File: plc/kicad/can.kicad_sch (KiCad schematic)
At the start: 1 part, among them CN2 DB2ERC-3.81-3P

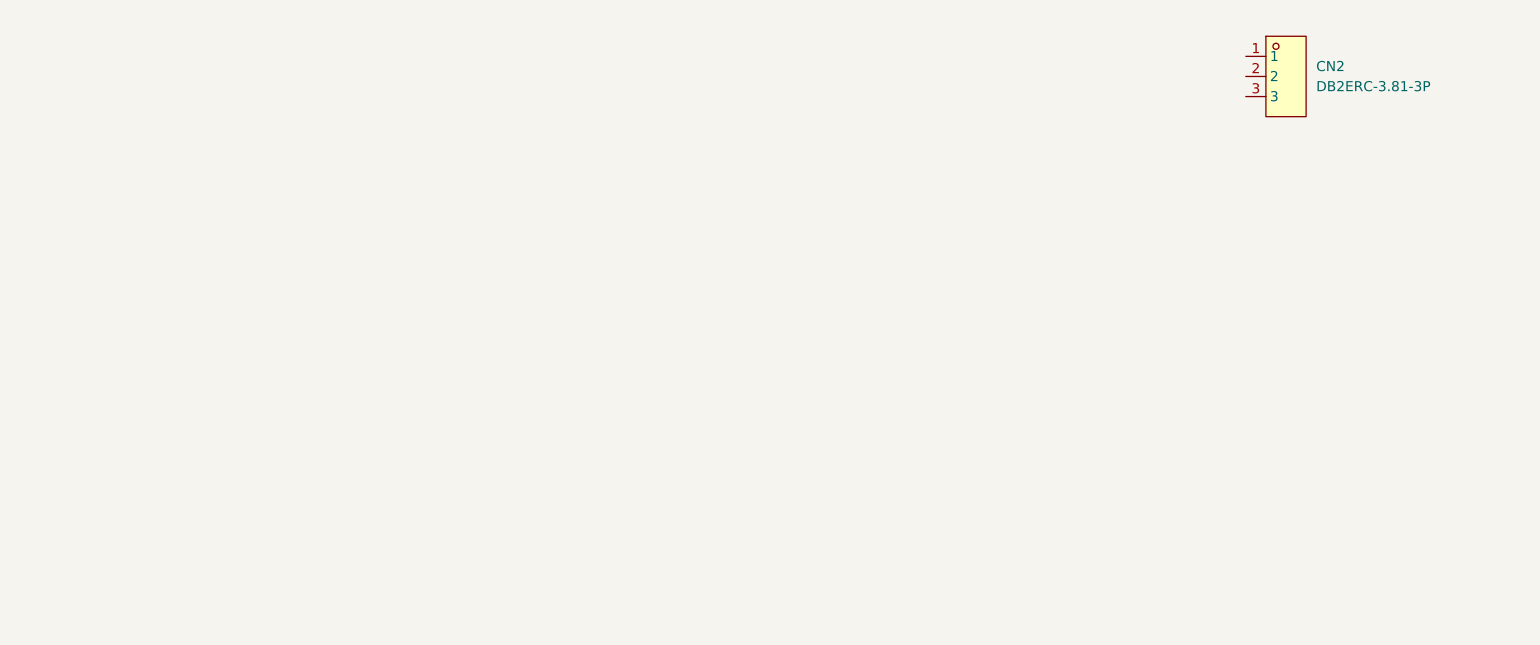
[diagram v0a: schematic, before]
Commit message: Added CAN circuit
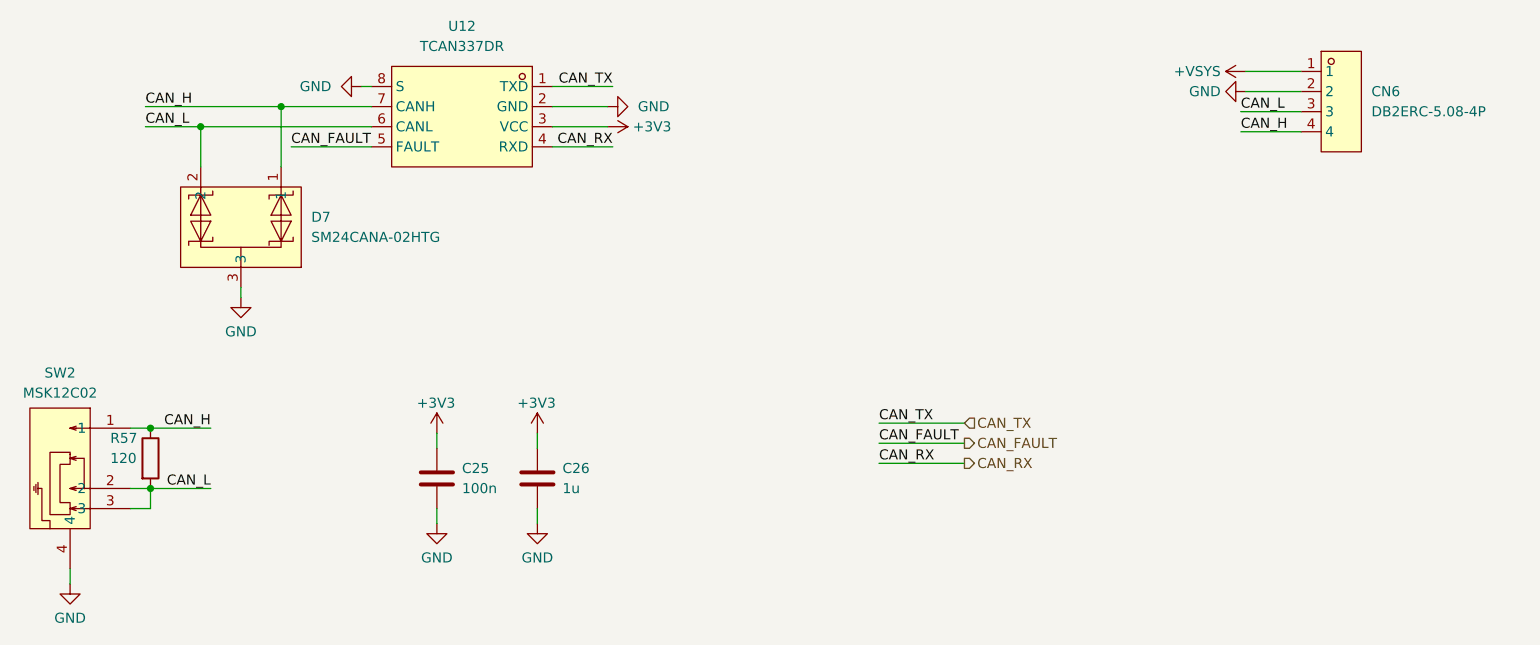
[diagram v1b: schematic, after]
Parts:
- removed CN2: DB2ERC-3.81-3P, LibrePLC32:CONN-TH_3P-P3.81_DB2ERC-3.81-3P, symbol LibrePLC32:DB2ERC-3.81-3P
- added C25: 100n, Capacitor_SMD:C_0805_2012Metric, symbol Device:C
- added C26: 1u, Capacitor_SMD:C_0805_2012Metric, symbol Device:C
- added CN6: DB2ERC-5.08-4P, LibrePLC32:CONN-TH_4P-P5.08_DB2ERC-5.08-4P, symbol LibrePLC32:DB2ERC-5.08-4P
- added D7: SM24CANA-02HTG, LibrePLC32:SOT-23_L2.9-W1.3-P1.90-LS2.4-BR, symbol LibrePLC32:SM24CANA-02HTG
- added R57: 120, Resistor_SMD:R_0805_2012Metric, symbol Device:R
- added SW2: MSK12C02, LibrePLC32:SW-TH_MSK12C02, symbol LibrePLC32:MSK12C02
- added U12: TCAN337DR, LibrePLC32:SOIC-8_L4.9-W3.9-P1.27-LS6.0-BL, symbol LibrePLC32:TCAN337DR
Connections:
- new net +3V3: C25.1, C26.1, U12.3 (VCC)
- new net +VSYS: CN6.1
- new net CAN_FAULT: U12.5 (FAULT)
- new net CAN_H: CN6.4, D7.1, R57.1, SW2.1, U12.7 (CANH)
- new net CAN_L: CN6.3, D7.2, R57.2, SW2.2, SW2.3, U12.6 (CANL)
- new net CAN_RX: U12.4 (RXD)
- new net CAN_TX: U12.1 (TXD)
- new net GND: C25.2, C26.2, CN6.2, D7.3, SW2.4, U12.2 (GND), U12.8 (S)
